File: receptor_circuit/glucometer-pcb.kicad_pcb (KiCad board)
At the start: 2 copper layers, 43.1 x 79.4 mm, 21 parts, among them IC1 RC4558IP, IC2 LM1458N, IC3 RC4558IP

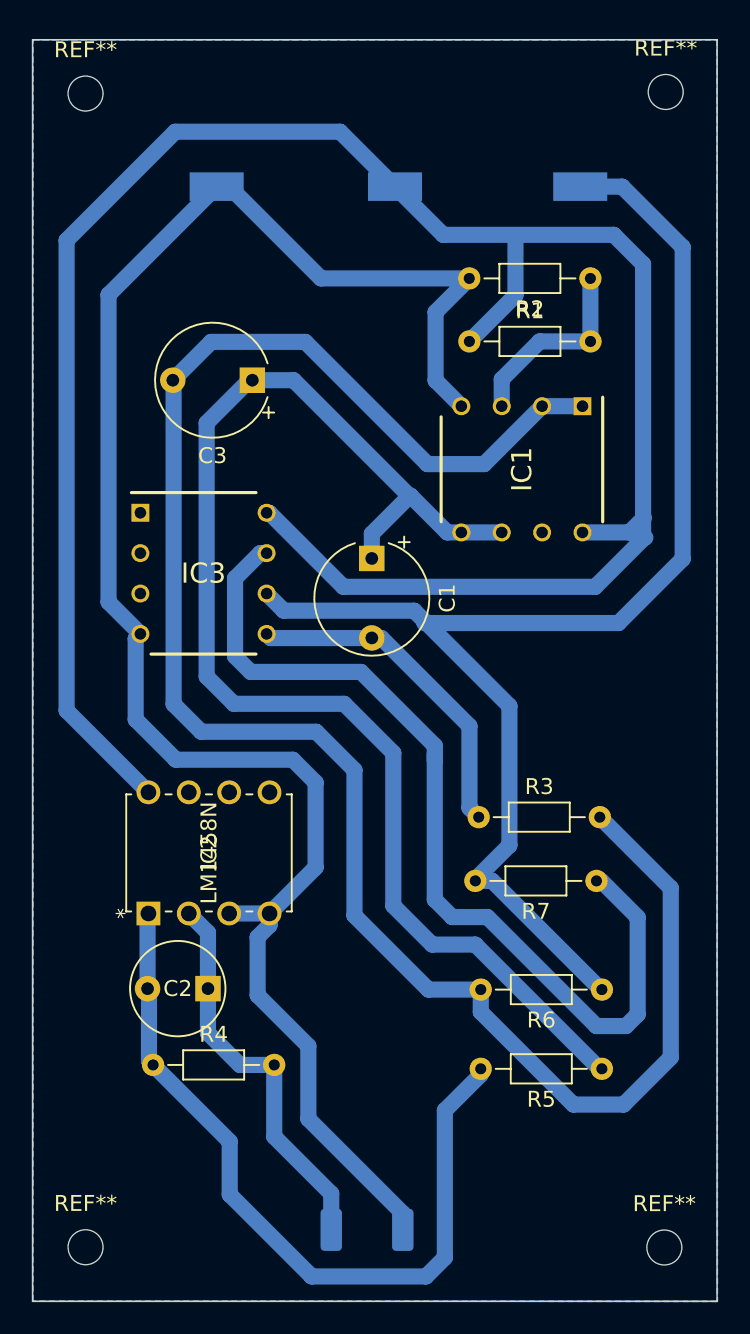
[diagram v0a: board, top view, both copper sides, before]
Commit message: fixed PCB
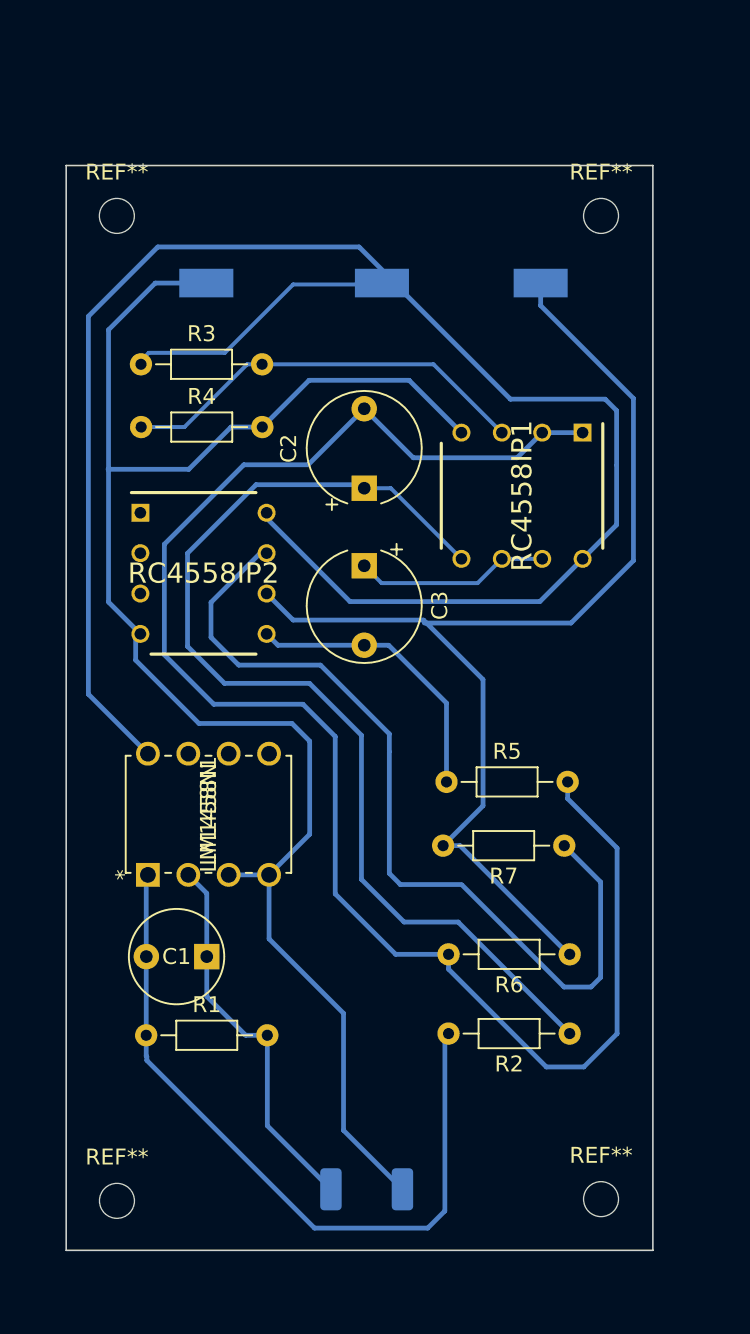
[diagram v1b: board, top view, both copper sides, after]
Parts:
- moved REF** 34.6 mm to (175.8, 173.0)
- moved REF** 32.6 mm to (206.3, 172.9)
- moved R4 29.8 mm to (177.3, 124.3), turned to 0 degrees
- moved R3 20.7 mm to (177.3, 120.4)
- moved C2 9.78 mm to (191.4, 128.2), turned to 90 degrees
- moved REF** 8.79 mm to (206.3, 111.1)
- moved REF** 7.94 mm to (175.8, 111.1)
- moved S_OUT1 6.56 mm to (202.5, 115.3)
- moved VCC1 6.12 mm to (192.5, 115.3)
- moved GND1 6.10 mm to (181.4, 115.3)
- moved R2 3.00 mm to (204.3, 162.5)
- moved R5 3.00 mm to (196.6, 146.7)
- moved R6 3.00 mm to (204.3, 157.5)
- moved R7 3.00 mm to (204.0, 150.7)
- moved RECEPTOR_DIODE1 2.55 mm to (191.5, 172.3)
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- renumbered C2 to C1, C3 to C2, C1 to C3, TP1 to GND1, IC2 to LM1458N1, R4 to R1, R5 to R2, R1 to R3, R2 to R4, R3 to R5, IC1 to RC4558IP1, IC3 to RC4558IP2, D1 to RECEPTOR_DIODE1, TP3 to S_OUT1, TP2 to VCC1
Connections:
- C3 pad 1: /SIGNAL_1 -> Net-(C3-Pad1)
- RC4558IP1 pad 6: /SIGNAL_1 -> Net-(C3-Pad1)
- RC4558IP1 pad 7: Net-(C1-Pad1) (its old number) -> Net-(C3-Pad1)
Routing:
- net /SIGNAL_1: track 85.2 -> 66.4 mm
- net /PWD_1.65: track 118.1 -> 102.4 mm
- net VCC: track 135.6 -> 119.9 mm
- net Net-(R3-Pad2): track 12.2 -> 26.1 mm
- net Net-(R6-Pad1): track 86.4 -> 72.7 mm
- net Net-(C3-Pad1): track 0.00 -> 12.3 mm
- net GND: track 113.5 -> 103.5 mm
- net Net-(R7-Pad1): track 58.6 -> 55.5 mm
- net /SIGNAL_2: track 21.1 -> 18.1 mm
- net Net-(C1-Pad2): track 48.8 -> 46.9 mm
- net Net-(C1-Pad1): track 24.9 -> 24.3 mm
- removed copper zone on B.Cu, net GND
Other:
- board size 43.1 x 79.4 mm -> 36.9 x 68.2 mm

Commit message: filled zone
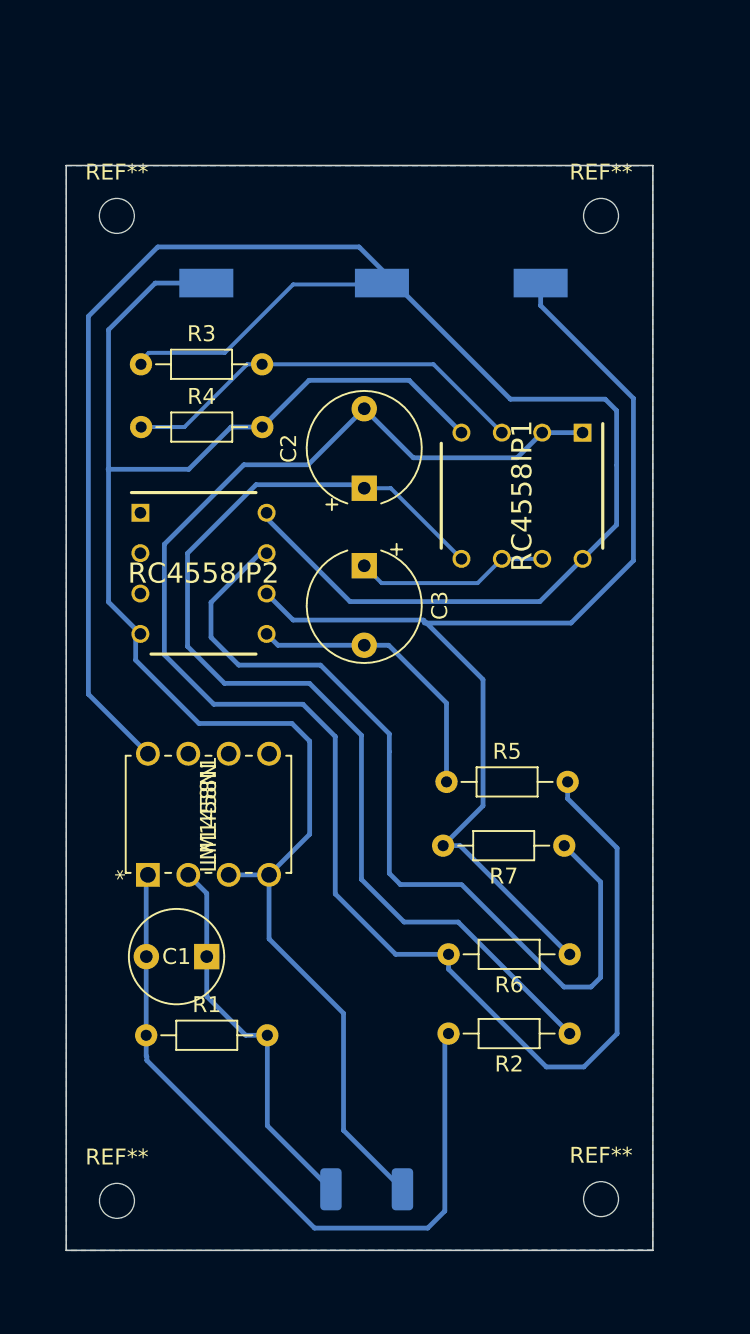
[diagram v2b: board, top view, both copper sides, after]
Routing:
- added copper zone on B.Cu, net GND
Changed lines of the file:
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@@
   (segment (start 200.031141 132.634489) (end 198.507094 134.158536) (width 0.25) (layer "B.Cu") (net 4))
   (segment (start 187.93263 140.464412) (end 182.583884 140.464412) (width 0.3) (layer "B.Cu") (net 5))
-  (segment (start 204.297807 162.49408) (end 197.284171 155.480444) (width 0.3) (layer "B.Cu") (net 5))
   (segment (start 204.297807 162.49408) (end 204.153157 162.49408) (width 0.3) (layer "B.Cu") (net 5))
   (segment (start 191.201485 143.733267) (end 187.93263 140.464412) (width 0.3) (layer "B.Cu") (net 5))
@@
   (segment (start 193.882535 155.478452) (end 191.201485 152.797402) (width 0.3) (layer "B.Cu") (net 5))
   (segment (start 197.306235 155.478452) (end 193.882535 155.478452) (width 0.3) (layer "B.Cu") (net 5))
+  (segment (start 204.297807 162.49408) (end 197.284171 155.480444) (width 0.3) (layer "B.Cu") (net 5))
   (segment (start 197.491141 132.634489) (end 193.046426 128.189774) (width 0.25) (layer "B.Cu") (net 5))
   (segment (start 205.187383 164.594522) (end 202.830187 164.594522) (width 0.3) (layer "B.Cu") (net 6))
@@
   (segment (start 205.641516 159.565867) (end 203.944052 159.565867) (width 0.3) (layer "B.Cu") (net 14))
   (segment (start 206.245698 158.961685) (end 205.641516 159.565867) (width 0.3) (layer "B.Cu") (net 14))
+  (zone (net 8) (net_name "GND") (layer "B.Cu") (hatch edge 0.508)
+    (connect_pads (clearance 0.508))
+    (min_thickness 0.254) (filled_areas_thickness no)
+    (fill yes (thermal_gap 0.508) (thermal_bridge_width 0.508))
+    (polygon
+      (pts
+        (xy 209.532853 107.900727)
+        (xy 209.53372 176.101312)
+        (xy 172.642584 176.140236)
+        (xy 172.631586 107.900294)
+      )
+    )
+  )
 )
